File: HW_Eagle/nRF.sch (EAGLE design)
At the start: 9 parts, among them X1 B4B-ZR

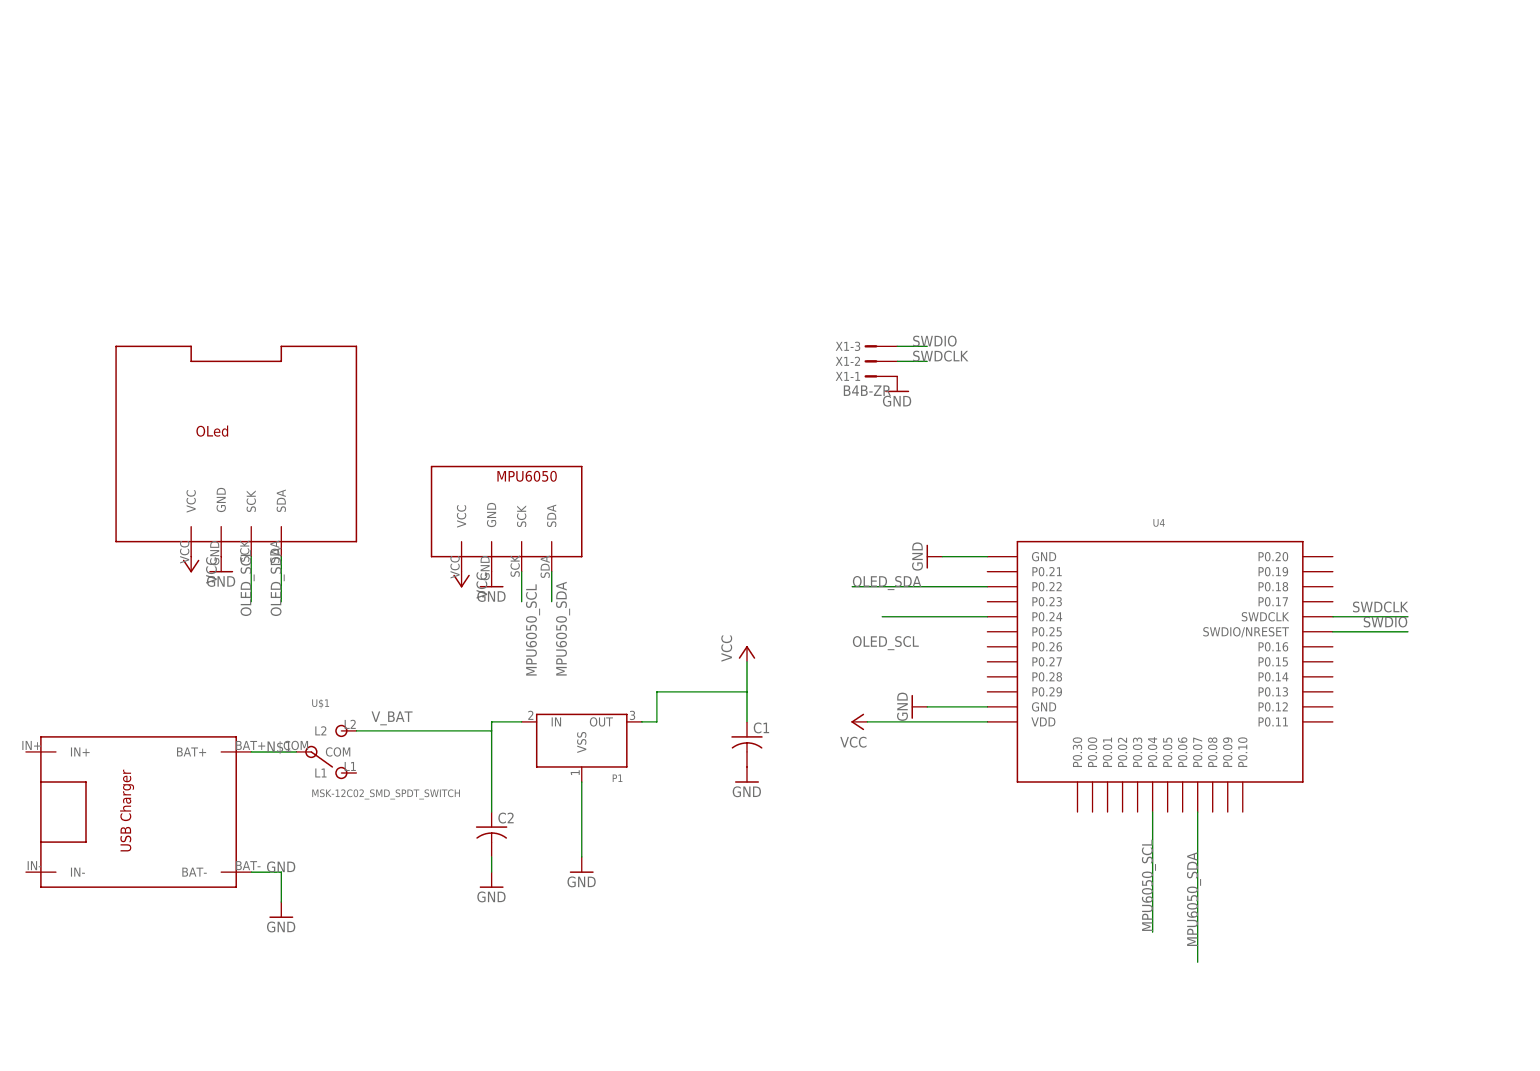
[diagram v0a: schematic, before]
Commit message: [HW] Update HW v1.2
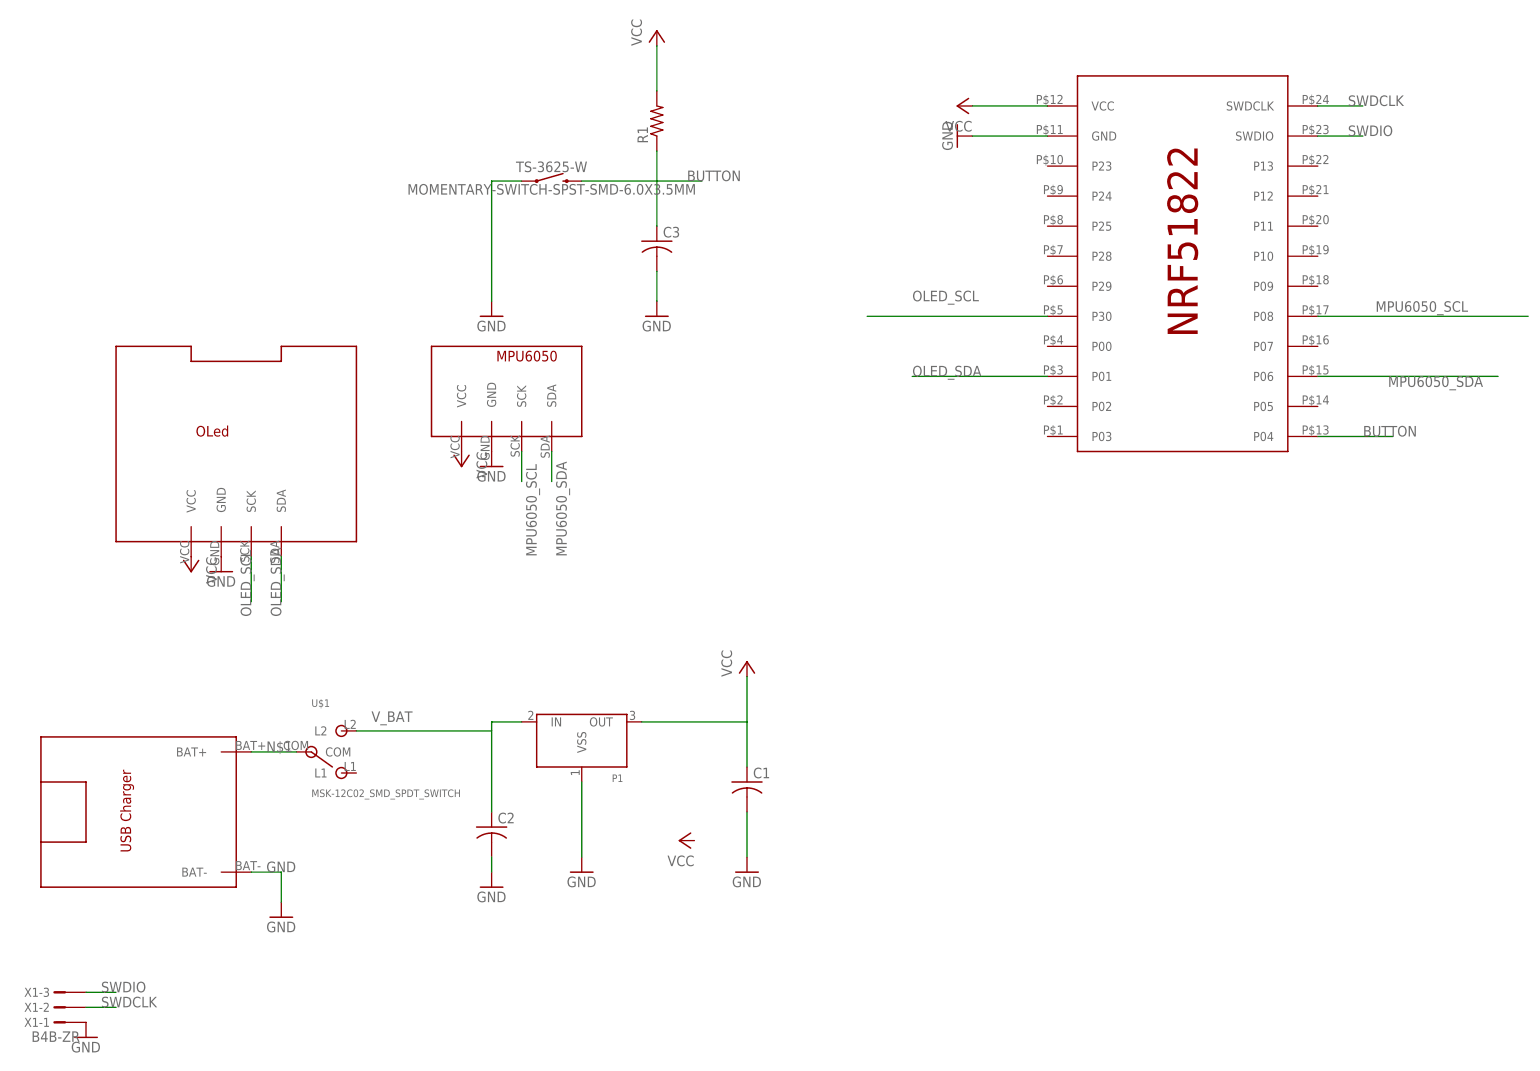
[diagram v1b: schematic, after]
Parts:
- removed U4: (no value), YJ-14015:YJ-14015
- added C3: (no value), rcl:C-USC0603
- added R1: (no value), rcl:R-US_R0603
- added TS-3625-W: MOMENTARY-SWITCH-SPST-SMD-6.0X3.5MM, SparkFun-Switches:MOMENTARY-SWITCH-SPST-SMD-6.0X3.5MM
- added U$5: NRF51822, nrf51822:NRF51822
- renumbered U$2 to U$6
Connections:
- new net BUTTON: C3.1, R1.1, TS-3625-W.2, U$5.P04
- net GND: now also C3.2, TS-3625-W.1, U$5.GND; no longer U4.GND@1, U4.GND@2
- net MPU6050_SCL: now also U$5.P08; no longer U4.P0.04
- net MPU6050_SDA: now also U$5.P06; no longer U4.P0.07
- net OLED_SCL: now also U$5.P30; no longer U4.P0.24
- net OLED_SDA: now also U$5.P01; no longer U4.P0.22
- net SWDCLK: now also U$5.SWDCLK; no longer U4.SWDCLK
- net SWDIO: now also U$5.SWDIO; no longer U4.SWDIO/NRESET
- net VCC: now also R1.2, U$5.VCC; no longer U4.VDD
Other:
- moved on the sheet: C1, X1-1, X1-2, X1-3
